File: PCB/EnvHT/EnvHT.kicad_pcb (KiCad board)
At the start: 2 copper layers, 29.5 x 18.3 mm, 25 parts, among them J1 DC, J2 DC, J4 Shelly, U1 LMR16006XDDCR, U2 QR, U4 ESP32-PICO-MINI-02, U7 SHT40

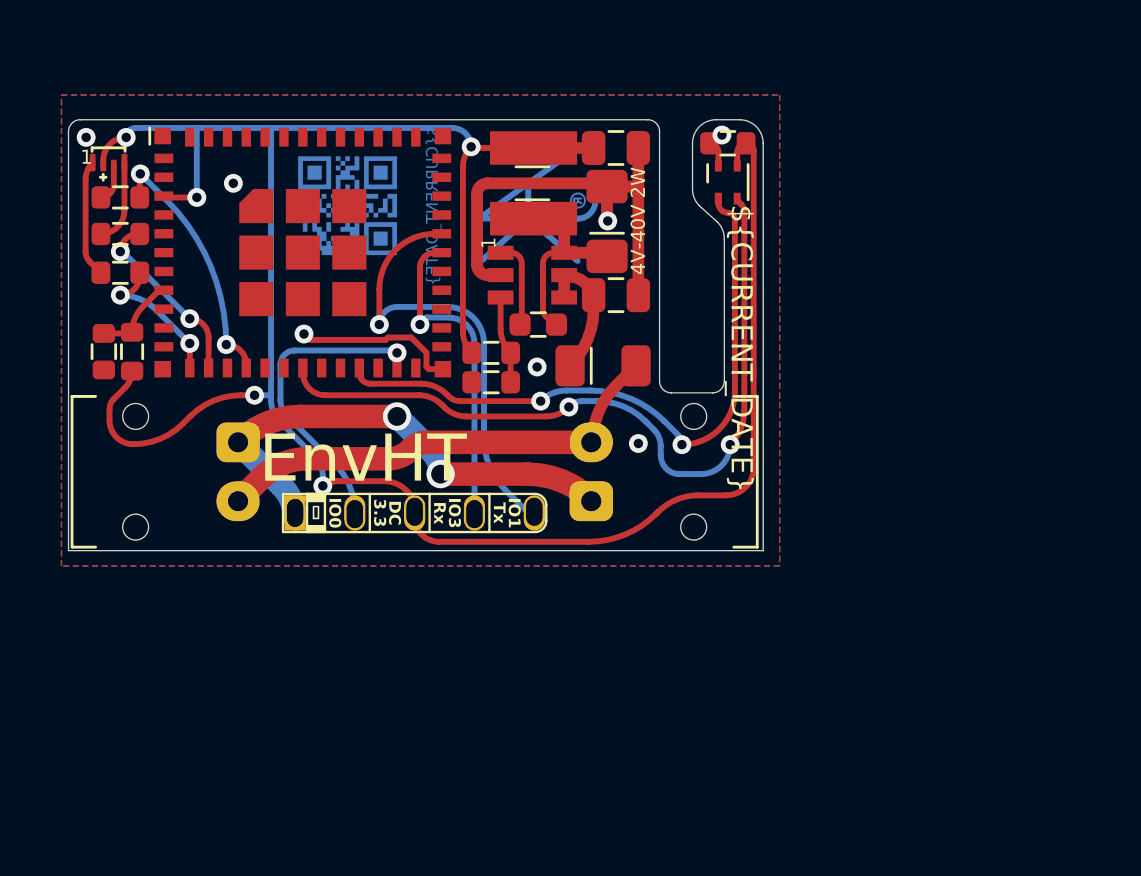
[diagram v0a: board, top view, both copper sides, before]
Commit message: Library update
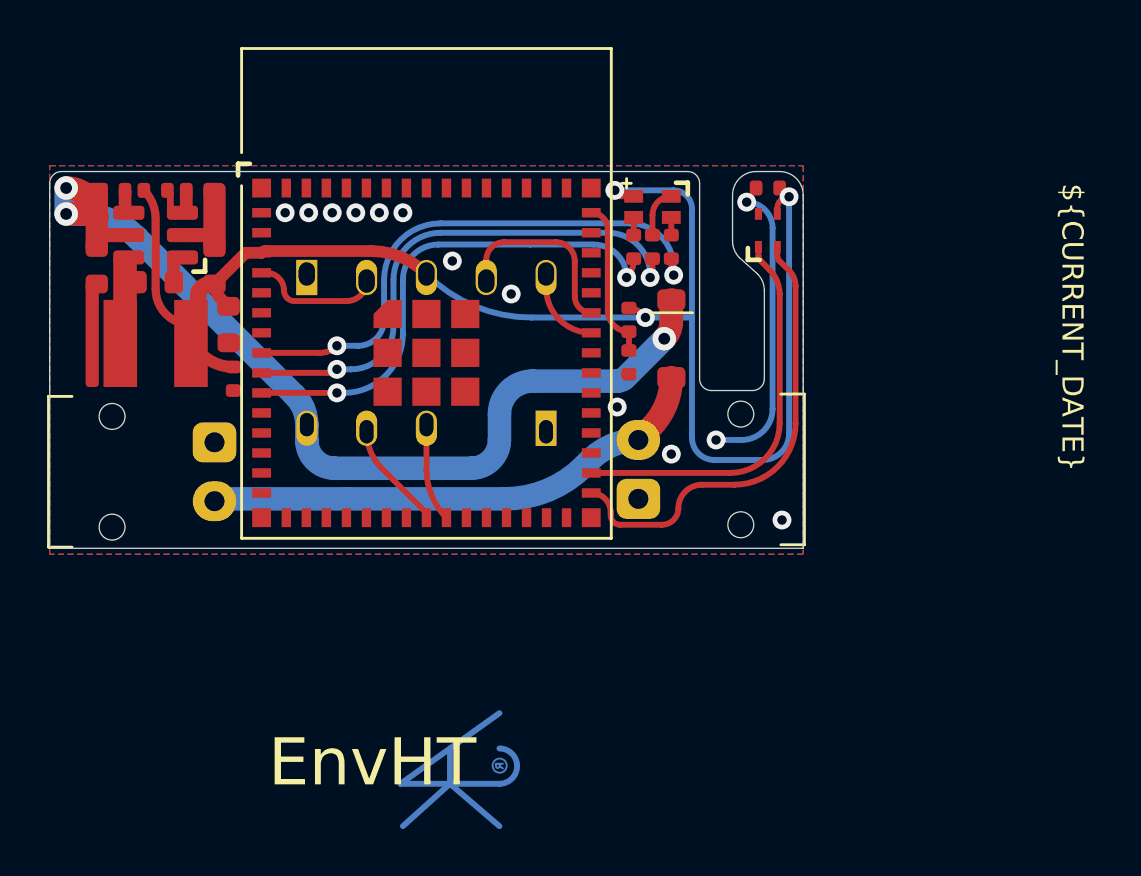
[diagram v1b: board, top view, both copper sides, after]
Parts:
- removed C5: 1uF, RevK:C_0603
- removed D2: D, RevK:D_1206
- removed D3: LED_BARG, RevK:MHS190RGBCT
- removed L1: 6.8uH, RevK:L_4x4_
- removed R12: 10k, RevK:R_0603
- removed R2: 30k 1%, RevK:R_0603
- removed R9: 100R, RevK:R_0603
- removed U2: QR, RevK:QR-ENVMON
- removed U4: ESP32-PICO-MINI-02, RevK:ESP32-PICO-MINI-02
- added C6: 10uF 50V, RevK:C_0603_, F.Cu at (89.0, 85.0)
- added C7: 10uF 6.3V, RevK:C_0603_, F.Cu at (94.0, 85.0)
- added C8: 100nF, RevK:C_0603_, F.Cu at (91.5, 85.7)
- added D4: RGB, RevK:LED-RGB-1.6x1.6, F.Cu at (112.6, 82.5)
- added J3: Shelly, RevK:Shelly, B.Cu at (103.0, 85.5)
- added L2: 10uH, RevK:L_4x4_, F.Cu at (91.5, 88.3)
- added R3: 680R, RevK:R_0402, F.Cu at (112.6, 84.2)
- added R4: 2K, RevK:R_0402, F.Cu at (113.4, 84.2)
- added R5: 220R, RevK:R_0402, F.Cu at (111.8, 84.2)
- added R6: 124k, RevK:R_0402_, F.Cu at (91.5, 81.8)
- added U3: MD8942, RevK:SOT-23-6-MD8942, F.Cu at (91.5, 83.7)
- C1: footprint RevK:C_0603_ -> RevK:C_0402
- C2: value 2.2uF -> 22uF; footprint RevK:C_0805_ -> RevK:C_0603
- C3: value 10uF -> 1uF; footprint RevK:C_0805_ -> RevK:C_0402
- C4: footprint RevK:C_0603 -> RevK:C_0402
- D1: value Schottky -> D; footprint RevK:D_1206_ -> RevK:D_SOD-123
- J4: value Shelly -> USB-PROG; footprint RevK:Shelly -> RevK:USB-PROG
- R1: value 100k 1% -> 10K; footprint RevK:R_0603 -> RevK:R_0402
- R7: value 300R -> 39k2; footprint RevK:R_0603 -> RevK:R_0402_
- R8: value 1K -> 1M; footprint RevK:R_0603 -> RevK:R_0402_
- U1: value LMR16006XDDCR -> ESP32-S3-MINI-1; footprint RevK:SOT-23-Thin-6-Reg -> RevK:ESP32-S3-MINI-1
- moved Logo1 24.2 mm to (104.0, 107.0)
- moved C2 16.5 mm to (94.6, 87.5), turned to -90 degrees
- moved C1 13.2 mm to (94.8, 89.8), turned to -90 degrees
- moved C3 9.12 mm to (111.6, 89.1), turned to -90 degrees
- moved R1 6.02 mm to (111.6, 87.3), turned to -90 degrees
- moved D1 5.68 mm to (113.4, 88.1), turned to -90 degrees
- moved U1 5.58 mm to (103.0, 88.7), turned to 0 degrees
- moved J4 3.63 mm to (103.0, 91.9), turned to 0 degrees
- moved R7 3.31 mm to (93.3, 81.8)
- moved U7 2.66 mm to (117.5, 83.5)
- moved C4 2.55 mm to (117.5, 81.7)
- moved J2 2.00 mm to (112.0, 93.7)
- moved R8 1.87 mm to (89.7, 81.8)
- moved J1 1.00 mm to (94.0, 93.8)
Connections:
- J1 pad 2: Net-(D2-A) -> Net-(D1-A)
- J2 pad 2: Net-(D2-A) -> Net-(D1-A)
- J4 pad 1: GND -> DC
- J4 pad 2: BOOT -> D-
- J4 pad 3: +3.3V -> D+
- J4 pad 4: I -> GND
- R1 pad 2: Net-(U1-FB) -> Net-(U1-EN)
- U1 pad 1: unconnected-(U1-CB-Pad1) -> GND
- U1 pad 3: Net-(U1-FB) -> +3.3V
- U1 pad 4: DC -> Net-(J3-0)
- U1 pad 5: DC -> unconnected-(U1-GPIO1-Pad5)
- U1 pad 7: +3.3V -> GND
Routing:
- net +3.3V: track 95.6 -> 57.1 mm, vias 5 -> 3
- net DC: track 4.20 -> 39.9 mm, vias 0 -> 3
- net Net-(D1-A): track 0.00 -> 21.8 mm
- net Net-(D2-A): track 19.7 -> 0.00 mm
- net O: track 19.3 -> 0.00 mm, vias 1 -> 0
- net GND: track 30.7 -> 12.5 mm, vias 9 -> 13
- net B: track 6.00 -> 21.5 mm
- net G: track 7.78 -> 23.2 mm
- net I: track 14.2 -> 0.00 mm, vias 1 -> 0
- net BOOT: track 13.4 -> 0.00 mm, vias 1 -> 0
- net SCL: track 32.1 -> 19.5 mm, vias 2 -> 0
- net R: track 10.7 -> 22.4 mm
- net SDA: track 27.1 -> 16.9 mm, vias 2 -> 0
- net Net-(J3-Rx): track 0.00 -> 8.05 mm
- net Net-(U1-EN): track 0.00 -> 6.70 mm
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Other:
- board size 29.5 x 18.3 mm -> 32 x 16 mm
- board text added: "A"
- board text added: "Envht.revk.uk"
- board text added: "RGB: 9/8/10"
- board text added: "SCL: 35 SDA: 36"
- board text removed: "SDA: 15 SCL: 14 RGB: 25/33/32"

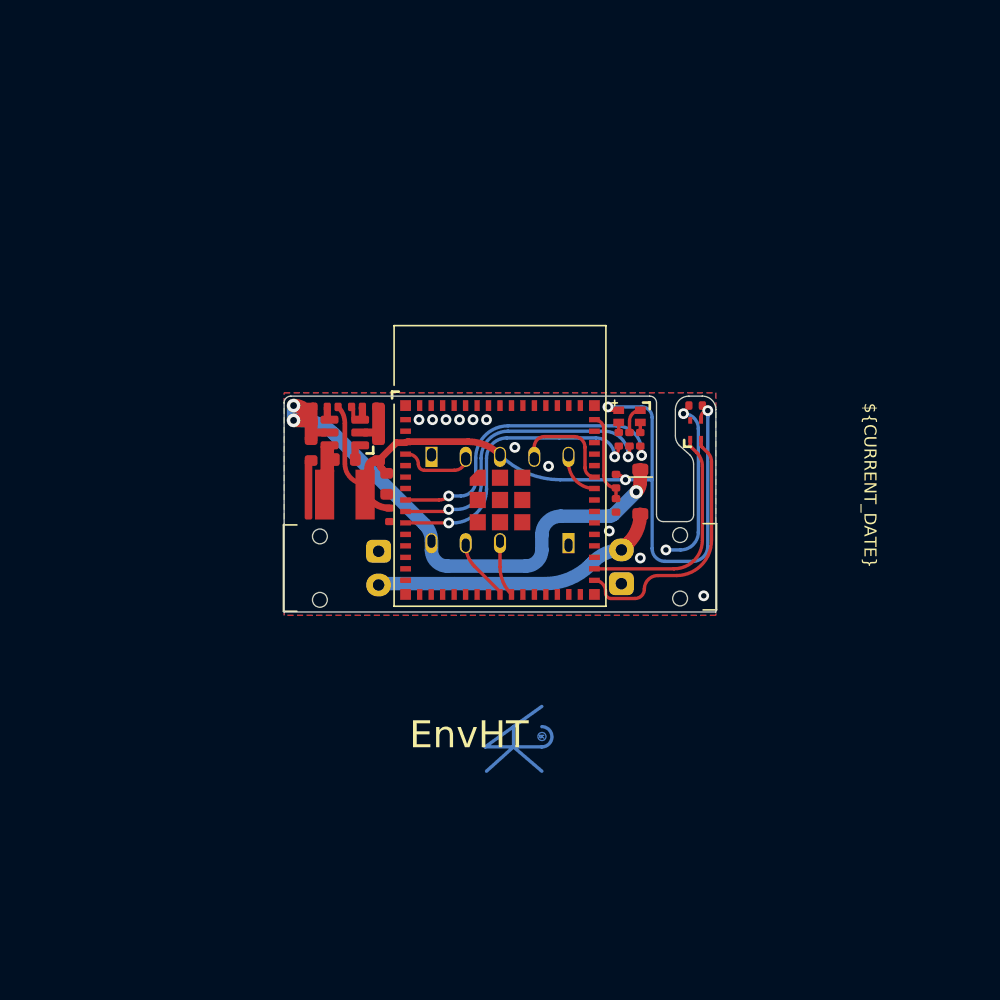
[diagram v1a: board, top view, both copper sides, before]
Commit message: Library update
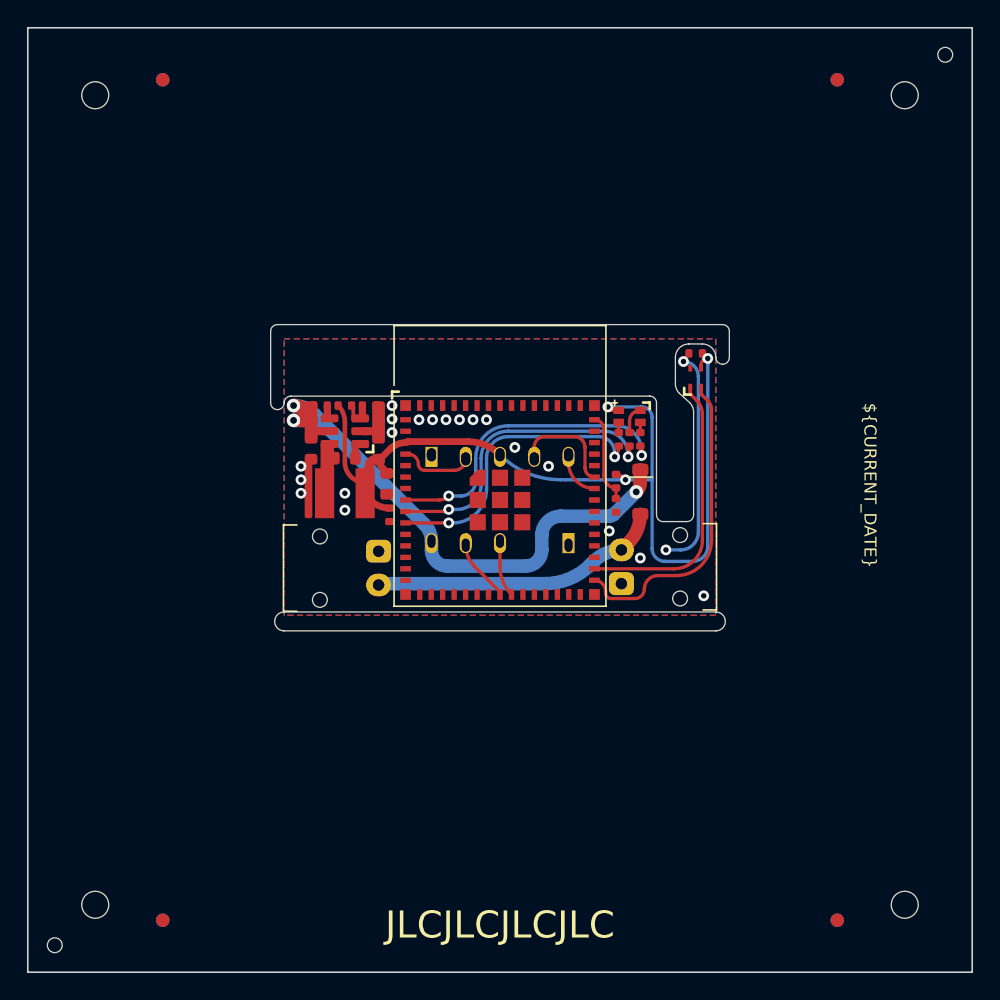
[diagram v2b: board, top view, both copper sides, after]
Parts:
- removed Logo1: AJK, RevK:AJK
- added PCB1: 70x70, RevK:PCB7070, F.Cu at (103.0, 88.7)
- added V2: ~, RevK:VCUT70, F.Cu at (87.0, 88.7)
- added V3: ~, RevK:VCUT70, F.Cu at (119.0, 88.7)
- moved C4 3.86 mm to (117.5, 77.8)
- moved U7 3.86 mm to (117.5, 79.6)
- moved S2 2.24 mm to (122.0, 86.0)
- moved S1 2.00 mm to (84.0, 86.0)
- moved C8 0.10 mm to (91.5, 85.6)
- moved U3 0.10 mm to (91.5, 83.6)
- moved C6 0.10 mm to (89.0, 84.9)
- moved C7 0.10 mm to (94.0, 84.9)
- moved L2 0.10 mm to (91.5, 88.2)
- moved R6 0.10 mm to (91.5, 81.7)
- moved R7 0.10 mm to (93.3, 81.7)
- moved R8 0.10 mm to (89.7, 81.7)
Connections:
- U1 pad 11: unconnected-(U1-GPIO7-Pad11) -> GND
- U1 pad 12: unconnected-(U1-GPIO8-Pad12) -> GND
- U1 pad 15: unconnected-(U1-GPIO11-Pad15) -> GND
- U1 pad 5: unconnected-(U1-GPIO1-Pad5) -> GND
- U1 pad 6: unconnected-(U1-GPIO2-Pad6) -> GND
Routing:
- net SCL: track 19.5 -> 23.4 mm
- net SDA: track 16.9 -> 20.8 mm
- net GND: track 12.5 -> 16.3 mm, vias 13 -> 21
- net +3.3V: track 57.1 -> 60.2 mm
- net DC: track 39.9 -> 42.6 mm
- net Net-(J3-Tx): track 3.52 -> 2.94 mm
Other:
- board size 32 x 16 mm -> 70 x 70 mm
- board text added: "5060634238106"
- board text removed: "EnvHT"
